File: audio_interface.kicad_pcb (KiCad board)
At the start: 2 copper layers, 36 x 32 mm, 28 parts, among them IC1 ATMEGA16U2, P1 USB_A, P2 AVR-ISP, P3 OUT, P4 EAR, Q1 BC849, Q2 BC849, Y1 CSTCE16M0V53MU

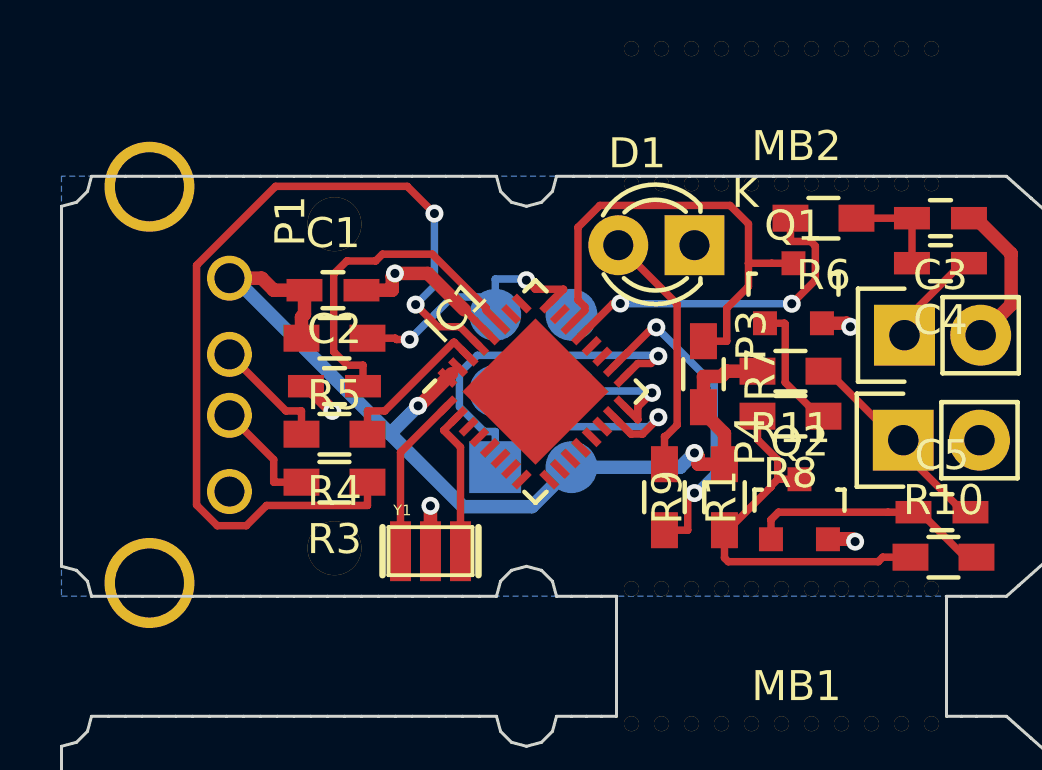
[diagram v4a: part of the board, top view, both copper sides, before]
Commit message: update
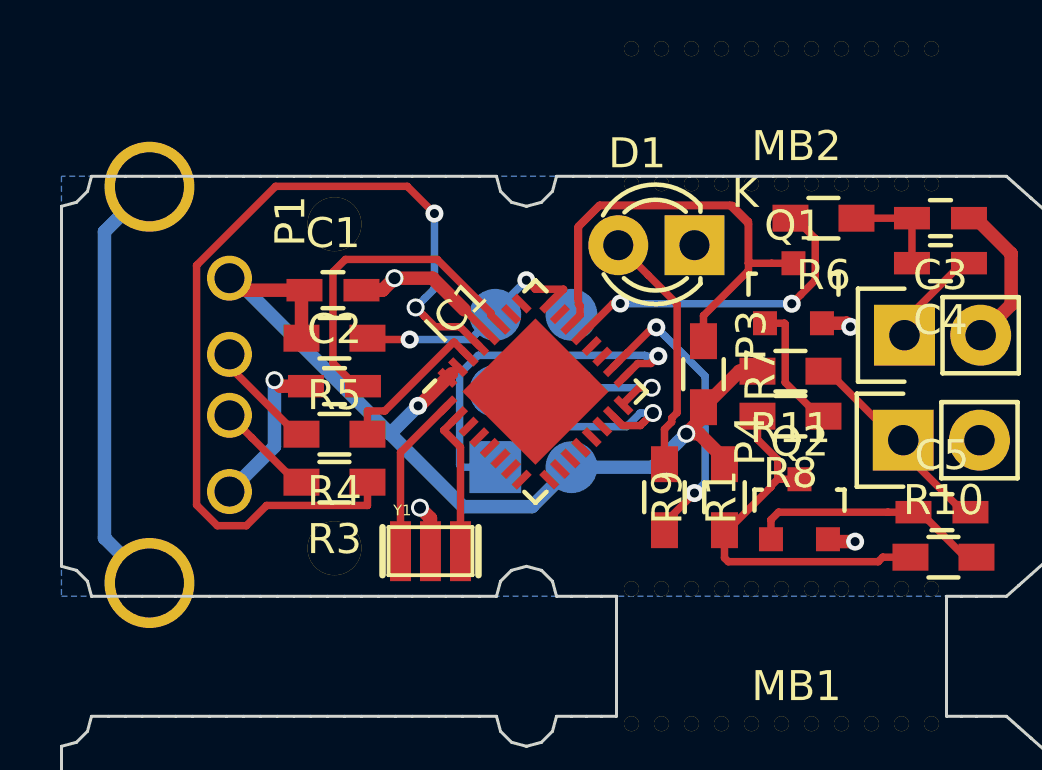
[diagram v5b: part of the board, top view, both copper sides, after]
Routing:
- net GND: track 16.3 -> 33.7 mm
- net PC7: track 16.3 -> 25.7 mm
- net +5V: track 33.3 -> 32.1 mm
- net SCK: track 8.29 -> 7.58 mm
- net PB4: track 10.7 -> 9.99 mm
- net MOSI: track 4.48 -> 3.95 mm

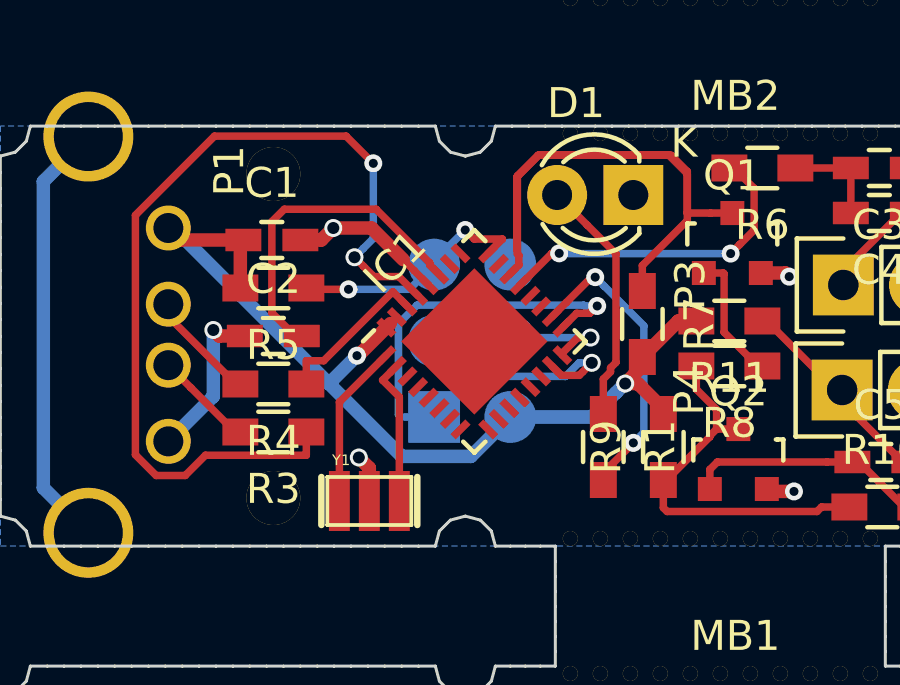
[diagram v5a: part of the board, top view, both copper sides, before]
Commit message: update
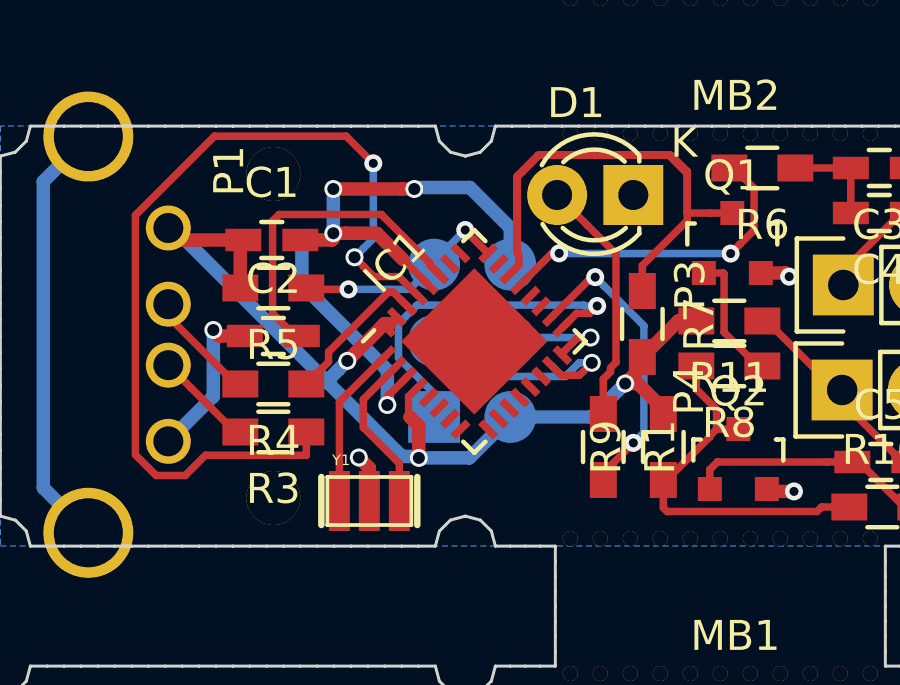
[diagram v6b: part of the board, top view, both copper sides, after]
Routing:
- net GND: track 33.7 -> 50.7 mm, vias 5 -> 8
- net +5V: track 32.1 -> 34.9 mm, vias 2 -> 3
- net ~RESET: track 8.89 -> 7.94 mm
- net MISO: track 12.6 -> 12.0 mm
- net Net-(IC1-Pad2): track 4.94 -> 5.47 mm

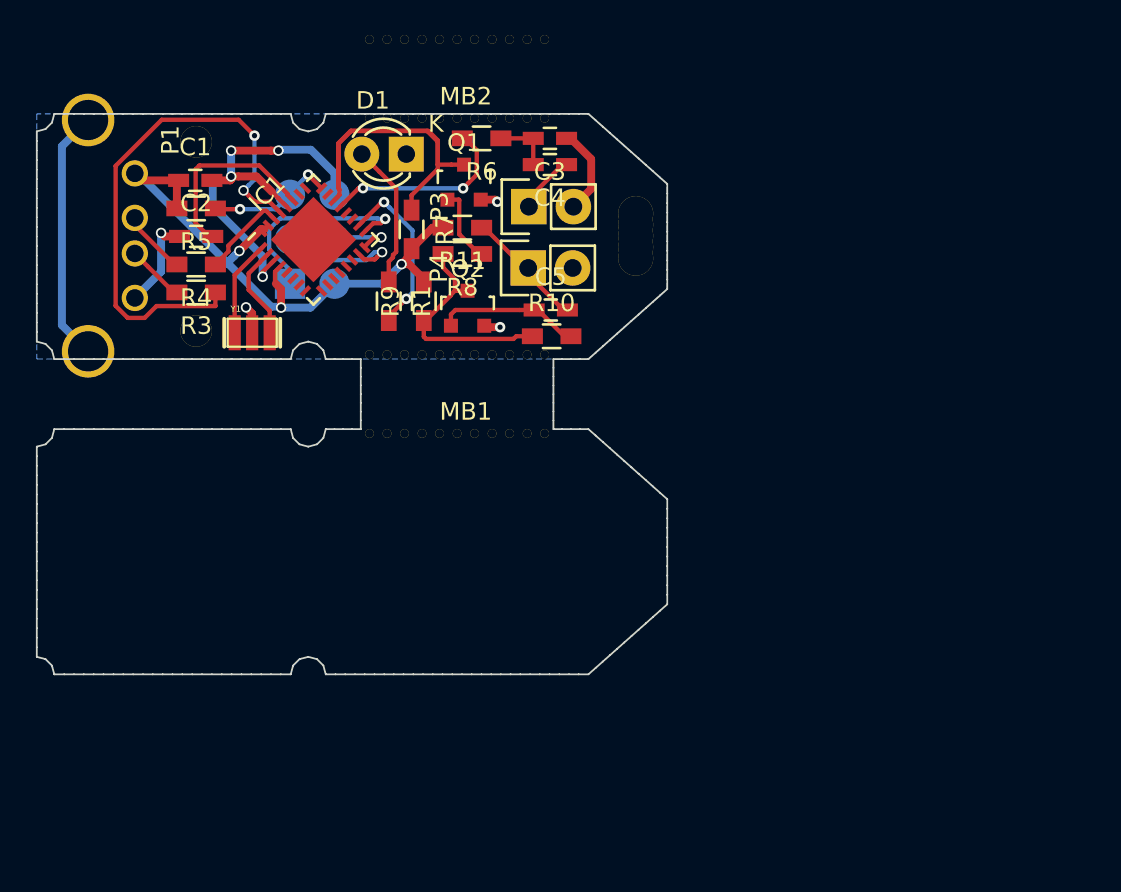
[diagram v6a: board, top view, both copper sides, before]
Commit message: Clean-up
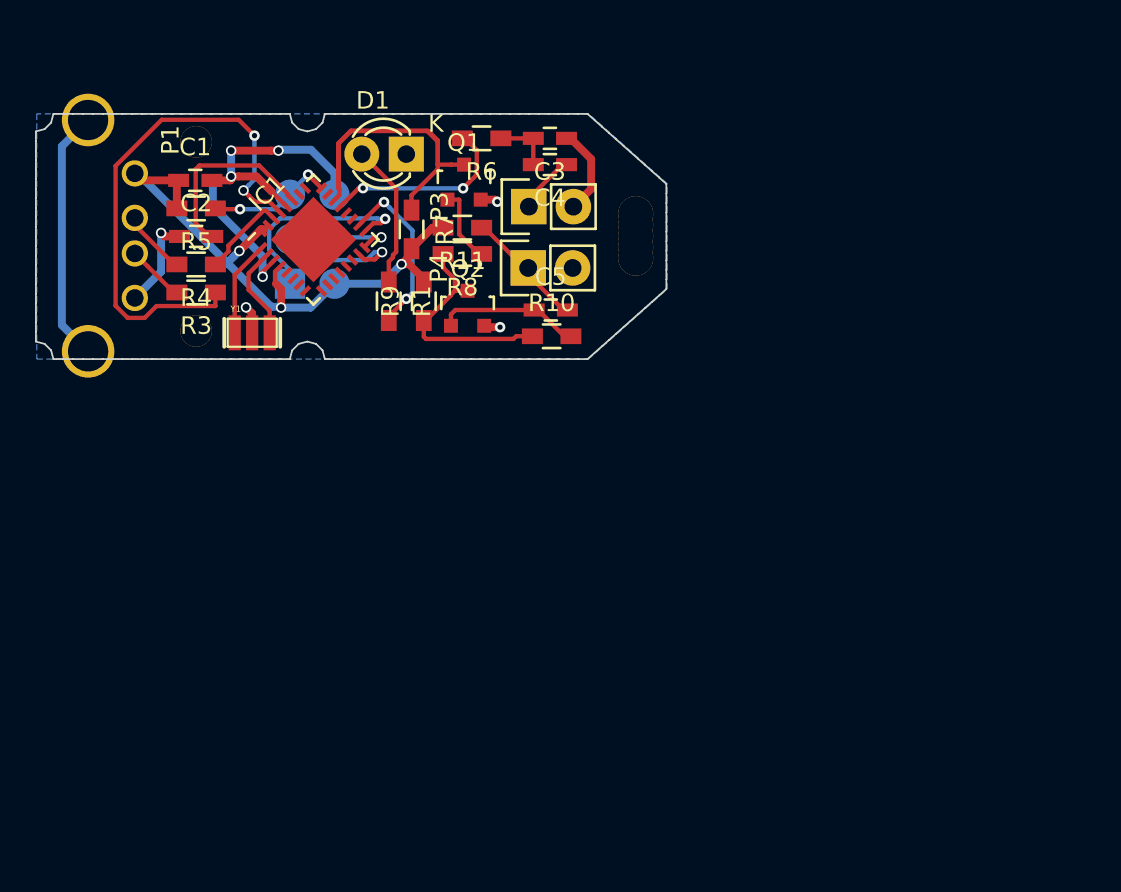
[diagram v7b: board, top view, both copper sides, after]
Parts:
- removed MB1, MB2: Mousebites, KaiBader:Mousebites
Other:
- board size 36 x 32 mm -> 36 x 14 mm
